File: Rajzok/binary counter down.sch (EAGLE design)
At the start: 17 parts, among them Q1 TP0602N2, Q2 TP0602N2, Q3 SUP75N06-08, Q4 SUP75N06-08

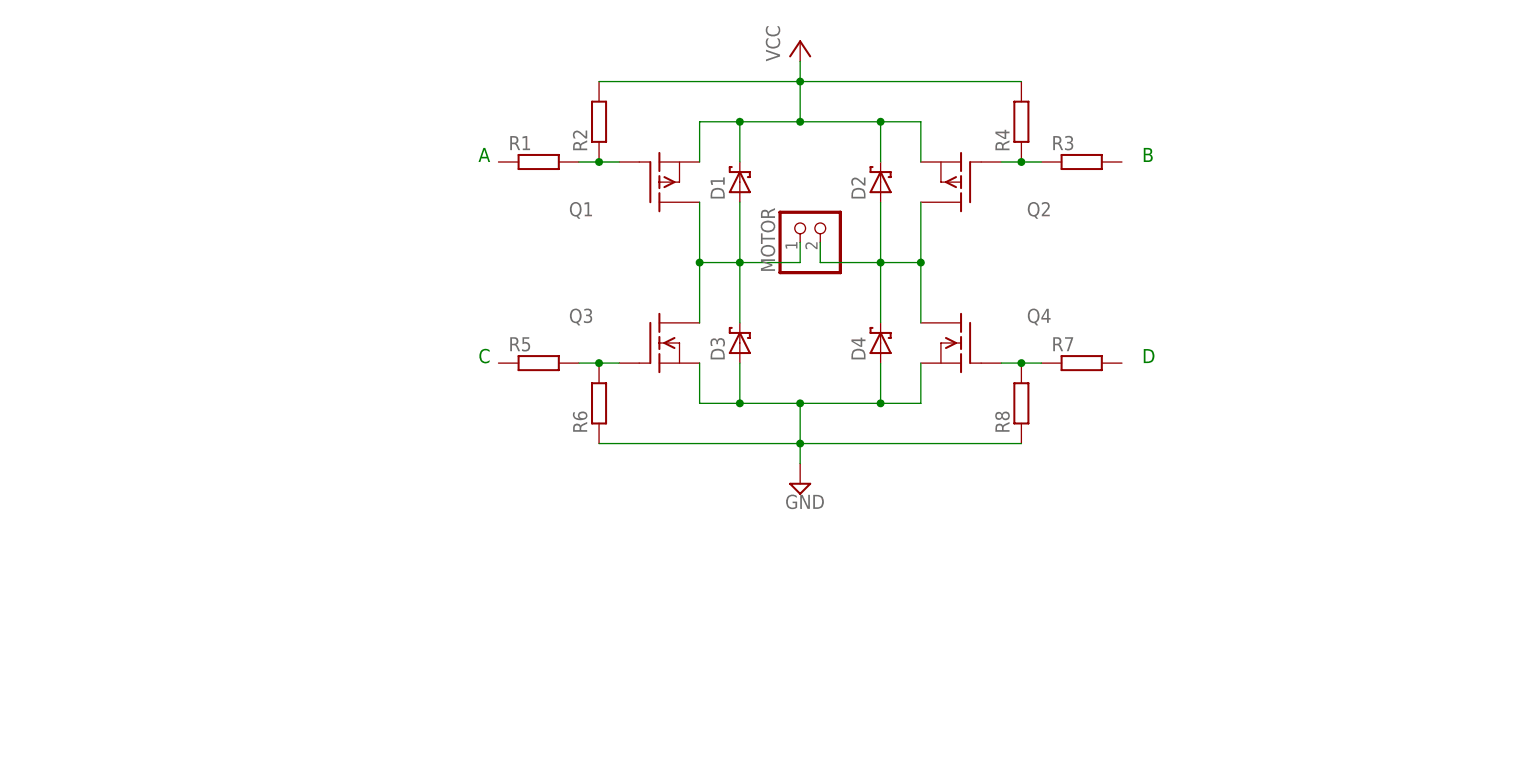
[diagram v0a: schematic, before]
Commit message: Rajzok 2017
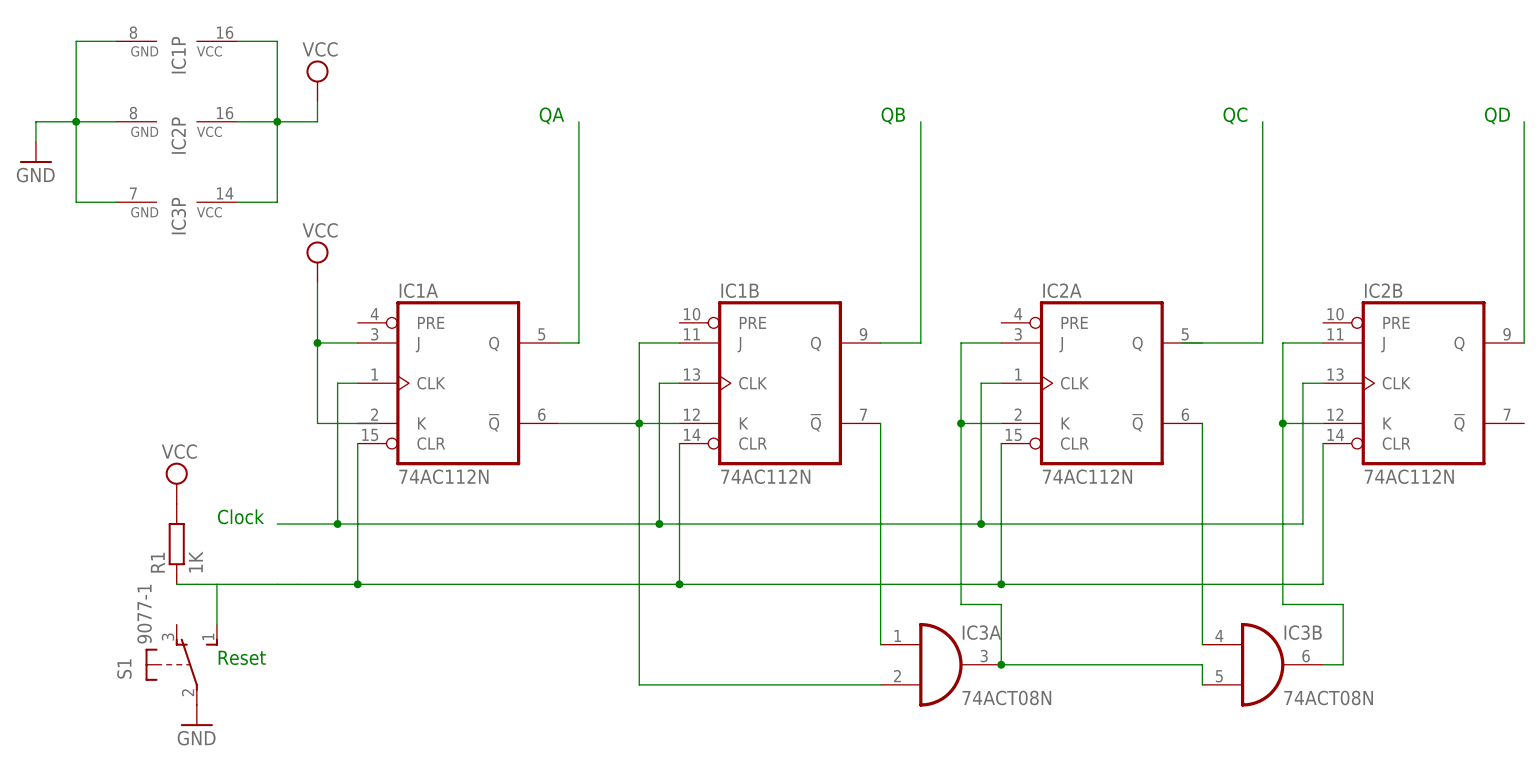
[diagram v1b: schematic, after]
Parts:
- removed D1, D2, D3, D4: 1N6267A, diode:1N6267A
- removed MOTOR: (no value), pinhead:PINHD-1X2
- removed Q1, Q2: TP0602N2, transistor-fet:TP0602N2
- removed Q3, Q4: SUP75N06-08, transistor-fet:SUP75N06-08
- removed R2, R3, R4, R5, R6, R7, R8: (no value), rcl:R-EU_0204/7
- added IC1, IC2: 74AC112N, 74xx-eu:74AC112N
- added IC3: 74ACT08N, 74xx-eu:74ACT08N
- added S1: 9077-1, switch-misc:9077-1
- R1: value (none) -> 1K
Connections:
- new net N$10: IC2A.!Q, IC3B.I0
- new net N$11: IC2B.J, IC2B.K, IC3B.O
- new net N$6: IC1A.CLR, IC1B.CLR, IC2A.CLR, IC2B.CLR, R1.1, S1.S
- new net N$8: IC2A.J, IC2A.K, IC3A.O, IC3B.I1
- net GND: now also IC1P.GND, IC2P.GND, IC3P.GND, S1.P; no longer D3.A, D4.A, Q3.S, Q4.S, R6.1, R8.1
- net N$1: now also IC1A.CLK, IC1B.CLK, IC2A.CLK, IC2B.CLK; no longer Q1.G, R1.2, R2.1
- net N$2: now also IC1A.!Q, IC1B.J, IC1B.K, IC3A.I1; no longer D2.A, D4.C, MOTOR.2, Q2.D, Q4.D
- net N$3: now also IC1A.Q; no longer Q2.G, R3.1, R4.1
- net N$4: now also IC1B.Q; no longer Q3.G, R5.2, R6.2
- net N$5: now also IC1B.!Q, IC3A.I0; no longer Q4.G, R7.1, R8.2
- net N$9: now also IC2B.Q; no longer D1.A, D3.C, MOTOR.1, Q1.D, Q3.D
- net VCC: now also IC1A.J, IC1P.VCC, IC2P.VCC, IC3P.VCC, R1.2; no longer D1.C, D2.C, Q1.S, Q2.S, R2.2, R4.2
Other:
- note added: "Clock"
- note added: "QA"
- note added: "QB"
- note added: "QC"
- note added: "QD"
- note added: "Reset"
- note removed: "A"
- note removed: "B"
- note removed: "C"
- note removed: "D"
- moved on the sheet: R1
